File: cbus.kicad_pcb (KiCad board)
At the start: 2 copper layers, 50 x 149 mm, 39 parts, among them CON1 AVR-JTAG-10, J1 CBUS_IO, J2 Conn_02x20_Odd_Even, J3 Conn_02x05_Top_Bottom, J4 Conn_02x05_Top_Bottom, U1 SN74LVC8T245DWR, U2 SN74LVC8T245DWR, U3 SN74LVC8T245DWR, U4 SN74LVC8T245DWR, U5 TPS76933, U6 ICE40HX1K-VQ100, U7 TPS76912, U8 AT25SF041-SSHD-B

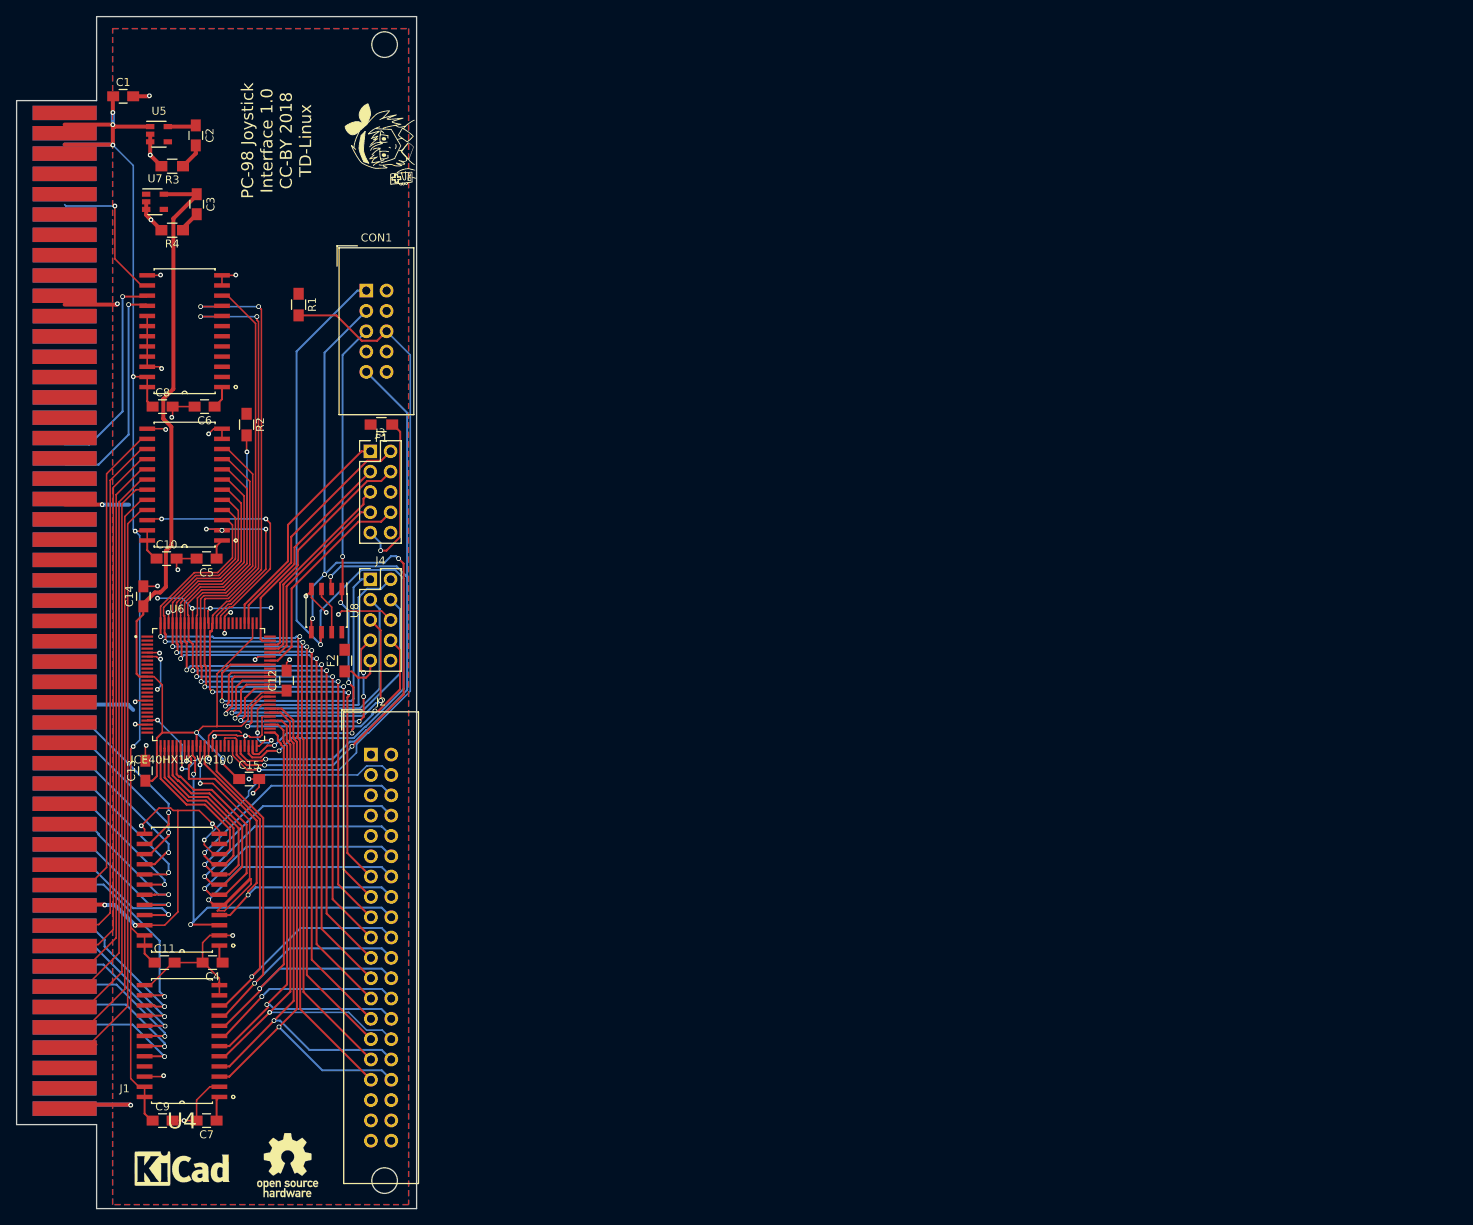
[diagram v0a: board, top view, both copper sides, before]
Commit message: Longboi
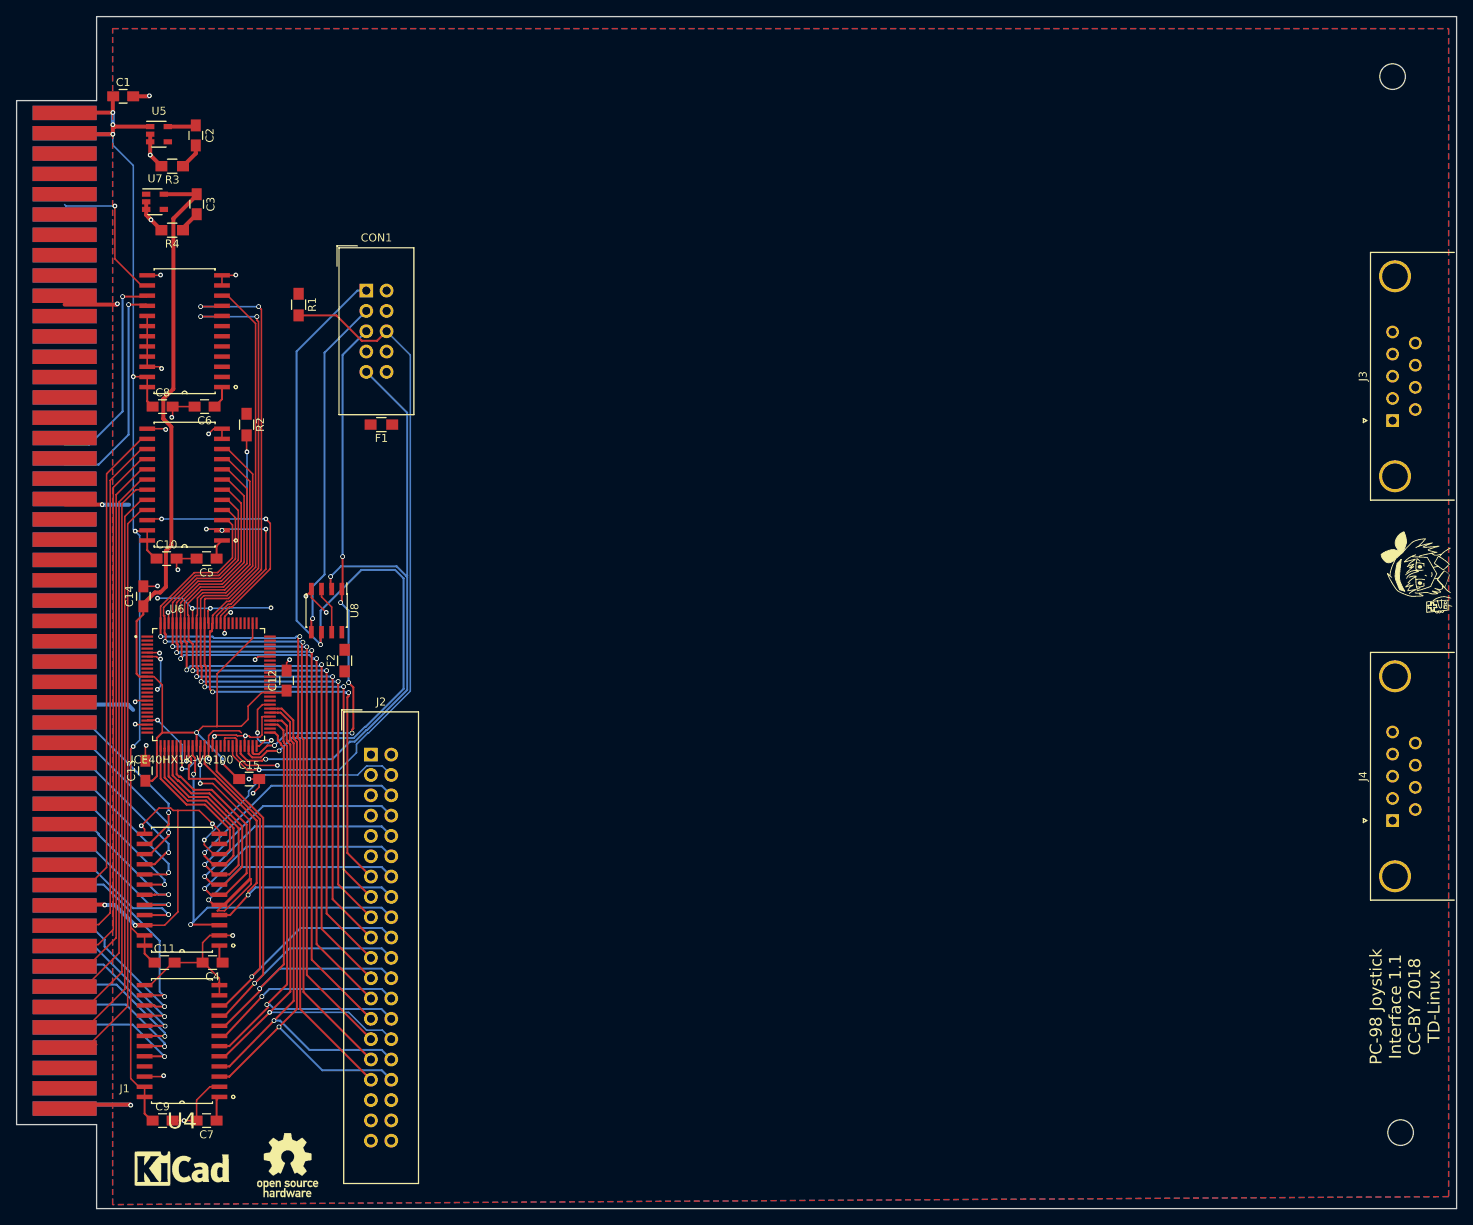
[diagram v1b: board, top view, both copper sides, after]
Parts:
- J3, J4: value Conn_02x05_Top_Bottom -> DB9_Male; footprint cbus:Pin_Header_Straight_2x05_Pitch2.54mm_Column_first -> Connector_Dsub:DSUB-9_Male_Horizontal_P2.77x2.84mm_EdgePinOffset4.94mm_Housed_MountingHolesOffset7.48mm
- moved svg2mod 140.1 mm to (204.0, 96.0)
- moved J4 131.3 mm to (201.0, 127.0), turned to 90 degrees
- moved J3 127.8 mm to (201.0, 77.0), turned to 90 degrees
- moved ? 127.1 mm to (202.0, 166.0)
- moved ? 126.1 mm to (201.0, 34.0)
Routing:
- net SDO: track 100.2 -> 53.2 mm, vias 5 -> 2
- net P2B: track 44.4 -> 0.00 mm, vias 1 -> 0
- net P2U: track 42.9 -> 0.00 mm, vias 1 -> 0
- net P2D: track 41.8 -> 0.00 mm, vias 1 -> 0
- net P2S: track 40.8 -> 0.00 mm, vias 1 -> 0
- net P2L: track 37.4 -> 0.00 mm, vias 2 -> 0
- net P2C: track 33.1 -> 0.00 mm, vias 2 -> 0
- net P2R: track 32.5 -> 0.00 mm, vias 4 -> 0
- net P1B: track 29.9 -> 0.00 mm
- net P1S: track 29.5 -> 0.00 mm
- net P1U: track 28.6 -> 0.00 mm
- net P1D: track 27.9 -> 0.00 mm
- net P1C: track 27.0 -> 0.00 mm
- net P1L: track 25.4 -> 0.00 mm
- net P1R: track 24.2 -> 0.00 mm
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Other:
- board size 50 x 149 mm -> 180 x 149 mm
- board text added: "PC-98 Joystick Interface 1.1 CC-BY 2018 TD-Linux"
- board text removed: "PC-98 Joystick Interface 1.0 CC-BY 2018 TD-Linux"
